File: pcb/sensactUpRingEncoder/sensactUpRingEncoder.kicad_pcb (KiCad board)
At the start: 2 copper layers, 45.7 x 39.5 mm, 66 parts, among them J2 IO35, J3 IO36, J32 PROG, J4 ToBase, J6 USB, Q1 IRLML0030, SW4 RESET, U1 ESP32-S3-MINI-1, U12 AHT20, U2 MAX98357A_WLP_Package, U4 AMS1117-3.3, U5 VCNL4040, U6 DS18B20U, U7 TJA1051TK-3, X1 Display_P169H002-CTP

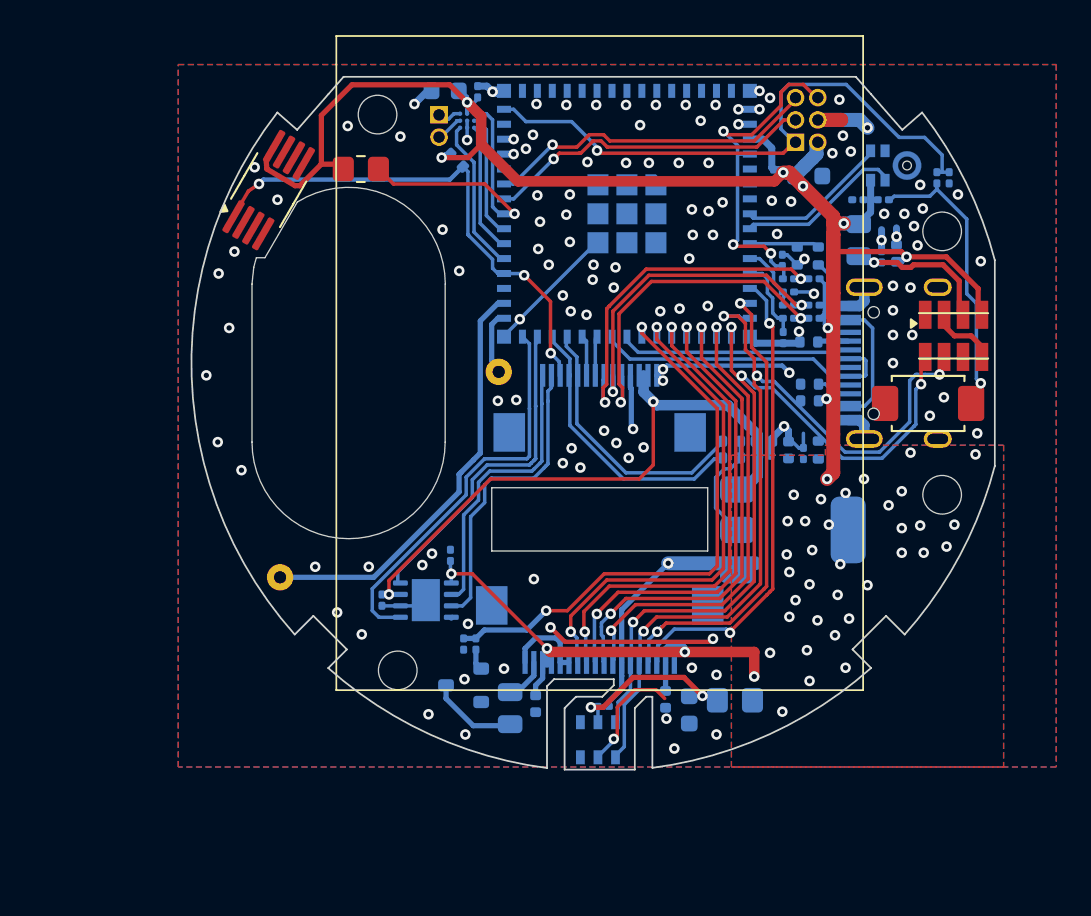
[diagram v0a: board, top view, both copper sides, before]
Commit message: Various improvements
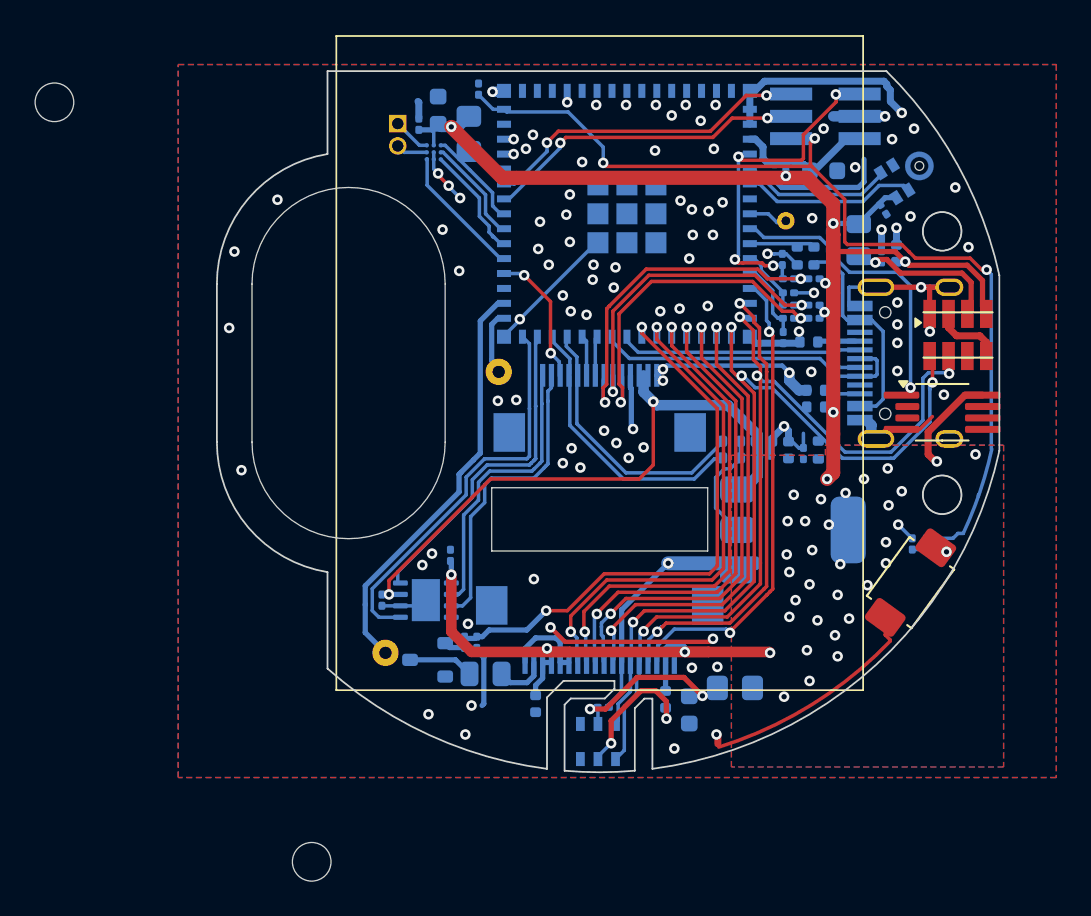
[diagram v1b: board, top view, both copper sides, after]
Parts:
- added J1: IO4, TestPoint:TestPoint_THTPad_D1.0mm_Drill0.5mm, B.Cu at (110.6, 91.9)
- J32: footprint Connector_PinHeader_1.27mm:PinHeader_2x03_P1.27mm_Vertical -> Connector_PinHeader_1.27mm:PinHeader_2x03_P1.27mm_Vertical_SMD
- R1: moved to B.Cu
- moved U6 40.4 mm to (119.5, 102.8), turned to 0 degrees
- moved C38 27.3 mm to (93.1, 84.4), turned to 90 degrees
- moved R46 21.8 mm to (113.2, 93.0), turned to 90 degrees
- moved R48 20.9 mm to (118.6, 110.3)
- moved R47 19.7 mm to (117.8, 110.3), turned to 90 degrees
- moved H4 18.4 mm to (69.0, 85.2)
- moved H3 12.0 mm to (83.6, 128.4)
- moved SW4 10.2 mm to (117.7, 112.5), turned to -126 degrees
- moved J3 7.38 mm to (87.8, 116.5)
- moved R1 6.47 mm to (92.5, 87.0), turned to -90 degrees
- moved C41 3.83 mm to (89.7, 86.4)
- moved U2 2.62 mm to (90.5, 88.0)
- moved Q1 2.51 mm to (90.2, 116.9)
- moved LS3 2.40 mm to (88.5, 86.4)
- moved R2 2.40 mm to (93.5, 117.7), turned to 0 degrees
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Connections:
- R46 pad 1: Onewire -> Onewire_intern
- U1 pad 5: unconnected-(U1-IO1-Pad5) -> MIC_DAT
- U1 pad 6: unconnected-(U1-IO2-Pad6) -> MIC_CLK
- U1 pad 8: MIC_DAT -> Net-(J1-Pin_1)
- U1 pad 9: MIC_CLK -> Onewire_intern
- U6 pad 1: Onewire -> Onewire_intern
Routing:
- net GND: track 81.2 -> 119.1 mm, vias 127 -> 102
- net Onewire: track 27.1 -> 7.77 mm, vias 3 -> 2
- net Onewire_intern: track 0.00 -> 16.9 mm, vias 0 -> 1
- net PROG_EN: track 34.2 -> 50.7 mm, vias 1 -> 3
- net Net-(R47-Pad1): track 15.3 -> 2.05 mm
- net AMP_SD: track 16.0 -> 5.65 mm, vias 1 -> 0
- net +3V3: track 127.4 -> 122.9 mm, vias 47 -> 43
- net Net-(J1-Pin_1): track 0.00 -> 2.30 mm
- net SDA: track 50.4 -> 48.1 mm
- net Net-(U5-LED_K): track 2.65 -> 4.07 mm
- net Net-(Q1-D): track 5.04 -> 3.72 mm
- net SCL: track 45.8 -> 46.9 mm
- net Net-(X1-LEDK): track 1.95 -> 2.97 mm
- net Net-(J6-VBUS-PadA4): track 11.4 -> 12.4 mm
- net PROG_TX: track 18.5 -> 19.5 mm, vias 1 -> 2
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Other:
- board size 45.7 x 39.5 mm -> 44.6 x 39.9 mm
